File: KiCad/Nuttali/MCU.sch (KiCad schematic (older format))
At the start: 19 parts

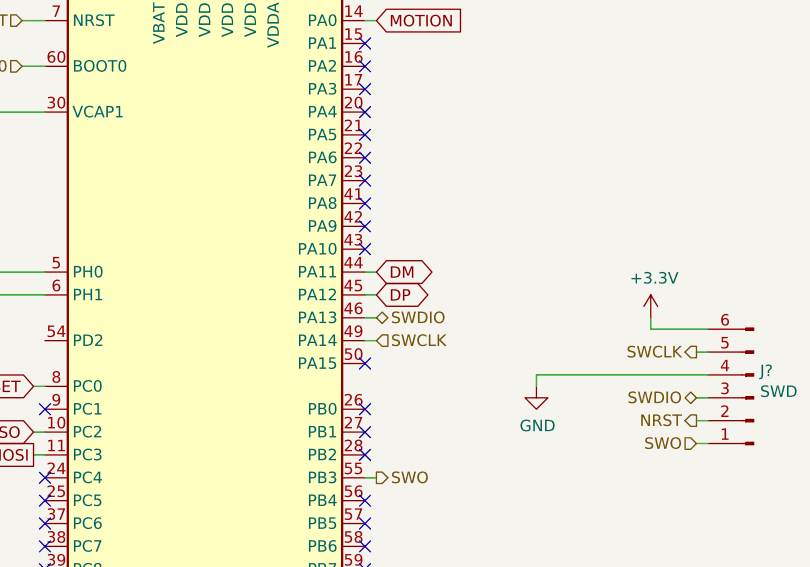
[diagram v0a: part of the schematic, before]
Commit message: Fixed power and USB
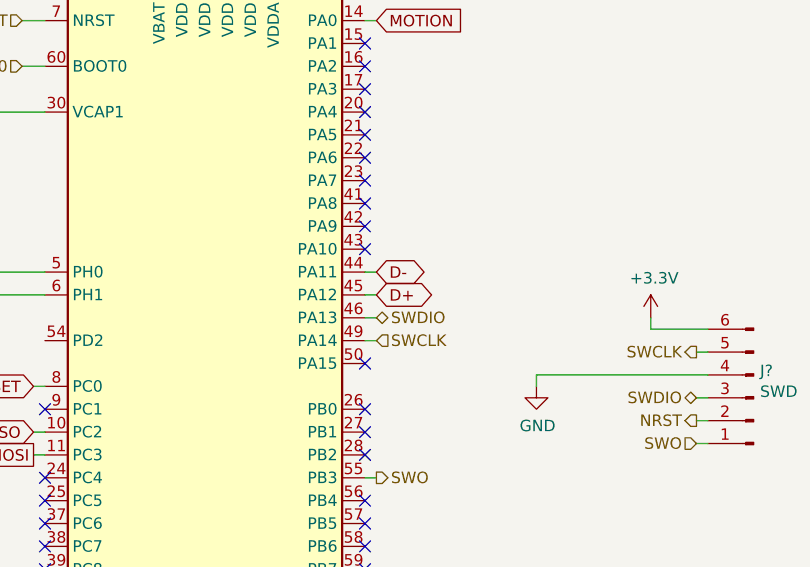
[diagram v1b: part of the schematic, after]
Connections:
- net DM renamed D-
- net DP renamed D+
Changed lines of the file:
@@
 	6200 2650 6150 2650
 Text GLabel 6200 3750 2    50   BiDi ~ 0
-DM
+D-
 Text GLabel 6200 3850 2    50   BiDi ~ 0
-DP
+D+
 Text GLabel 6200 5350 2    50   Output ~ 0
 SCK
